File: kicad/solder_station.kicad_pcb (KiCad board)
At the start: 2 copper layers, 31 parts, among them IC1 OPA336U, P2 POWER, P3 MCU, P4 KEYPAD, P5 JACK, Q1 PSMN*R*, Q2 PSMN*R*, SW1 SPST, SW2 SPST, SW3 SPST, SW4 SPST, T3 BSN20, U1 arduino_mini, U2 ROE-0505S

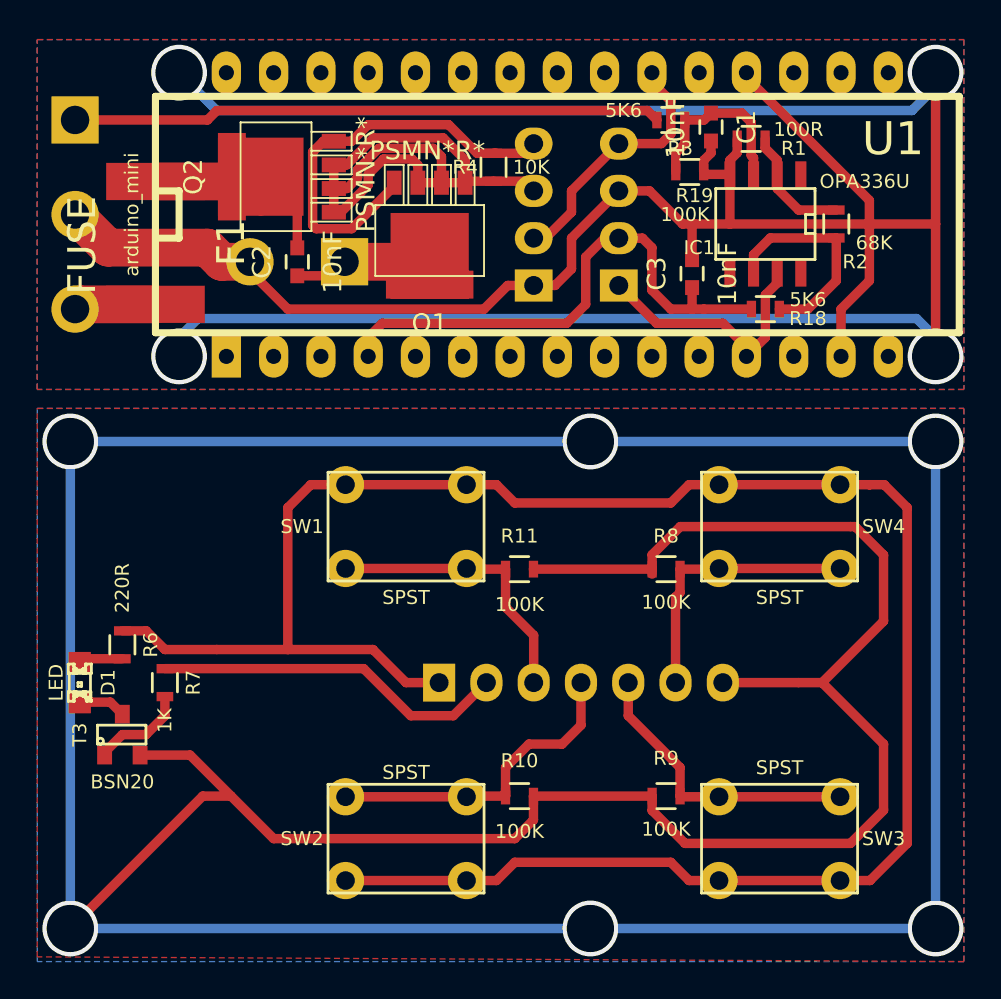
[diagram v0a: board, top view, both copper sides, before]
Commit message: Update kicad project
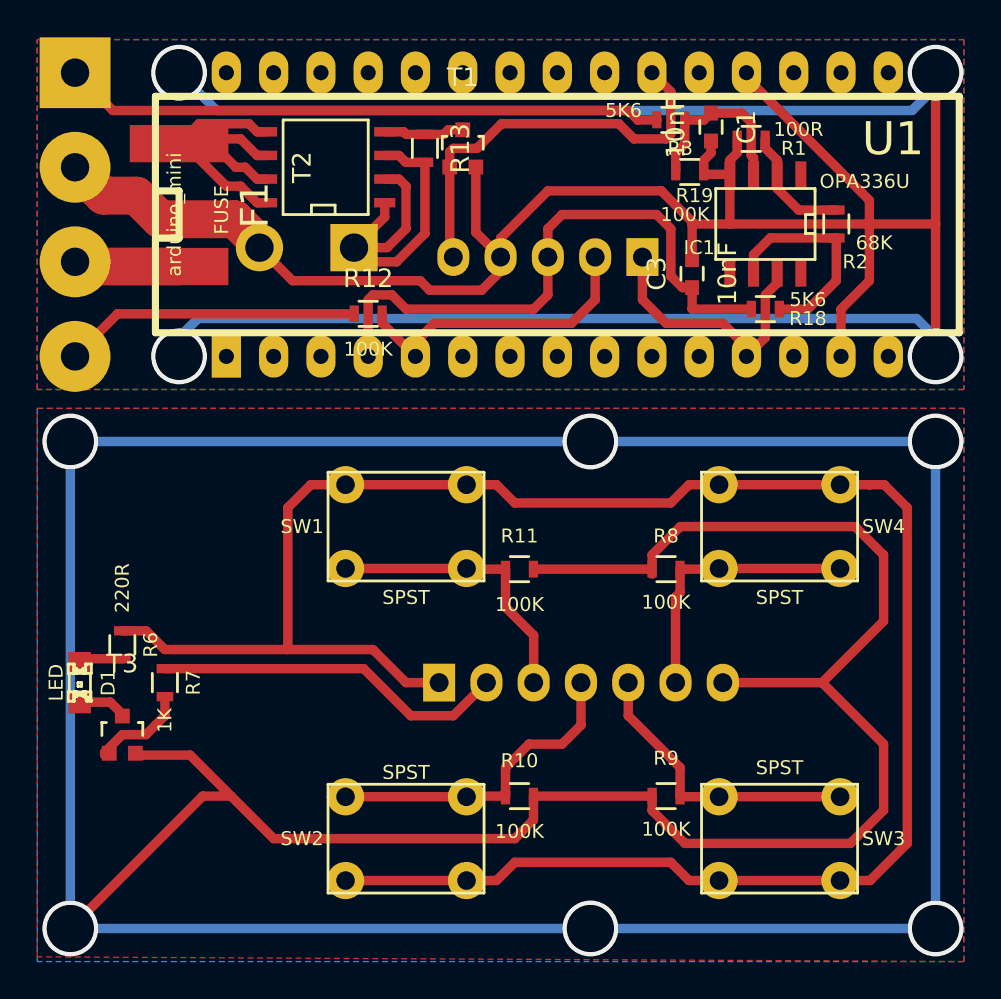
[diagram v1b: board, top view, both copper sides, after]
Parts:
- removed C2: 10nF, Capacitors_SMD:C_0603
- removed Q1, Q2: PSMN*R*, footprint:LFPAK-4
- removed R4: 10K, Resistors_SMD:R_0603
- removed U2: ROE-0505S, Pin_Headers:Pin_Header_Straight_1x04
- added R12: 100K, Resistors_SMD:R_0603, F.Cu at (142.0, 101.1)
- added R13: 10K, Resistors_SMD:R_0603, F.Cu at (145.0, 92.2)
- added T1: BSN20, Diodes_SMD:Diode_SOT23, F.Cu at (147.1, 92.2)
- added T2: IRF7476, SMD_Packages:SOIC-8-N, F.Cu at (139.7, 93.2)
- P3: footprint Pin_Headers:Pin_Header_Straight_1x04 -> Pin_Headers:Pin_Header_Straight_1x05
- P5: footprint Connect:bornier3 -> Connect:bornier4
- T3: footprint SMD_Packages:SOT-23 -> Diodes_SMD:Diode_SOT23
- moved P3 2.62 mm to (156.7, 98.0)
- moved F1 2.40 mm to (131.8, 95.2)
- moved P2 0.92 mm to (138.7, 97.5)
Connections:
- P3 pad 2: MCU_SENSOR -> MCU_STANDBY
- P3 pad 3: GND -> MCU_SENSOR
- P3 pad 4: MCU_HEATER -> GND
- U1 pad 5: Net-(U1-Pad5) -> MCU_STANDBY
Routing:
- net Net-(Q1-PadS): track 34.5 -> 0.00 mm
- net Net-(Q1-PadG): track 22.9 -> 0.00 mm
- net MCU_STANDBY: track 0.00 -> 16.7 mm
- net STANDBY: track 0.00 -> 15.9 mm
- net +12V: track 7.56 -> 20.5 mm
- net Net-(F1-Pad1): track 12.3 -> 22.9 mm
- net MCU_HEATER: track 16.0 -> 23.7 mm
- net GND: track 183.5 -> 190.6 mm
- net Net-(R13-Pad1): track 0.00 -> 4.35 mm
- net MCU_SENSOR: track 29.4 -> 32.8 mm
- net HEATER: track 4.42 -> 5.69 mm
- net +5V: track 13.9 -> 14.6 mm
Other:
- board text added: "SB"
